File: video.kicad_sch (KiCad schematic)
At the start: 22 parts, among them J2 DIN-7 Video, J3 DIN-5 Audio, J4 DIN-5 Power, Q1 BC547B, Q3 BC547B, Q4 BC547B, Q5 BC547B, Q6 BC547B

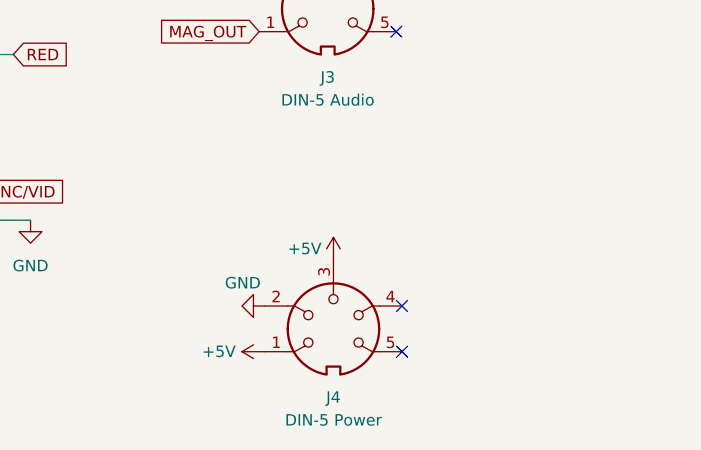
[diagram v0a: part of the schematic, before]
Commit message: Version 1.2 update
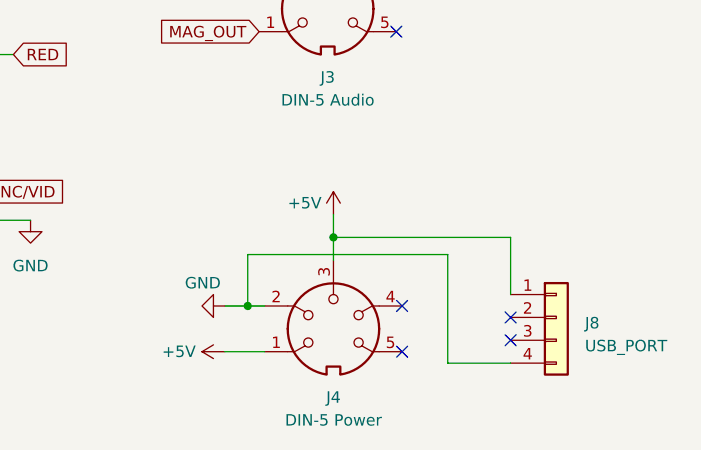
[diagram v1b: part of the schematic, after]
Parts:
- added J8: USB_PORT, Connector_PinHeader_2.54mm:PinHeader_1x04_P2.54mm_Vertical, symbol Connector_Generic:Conn_01x04
- J2: footprint w_conn_av:DIN-7-Variable -> Delta_sm_lib:DIN-7-Variable
- J3, J4: footprint w_conn_av:DIN-5-Variable -> Delta_sm_lib:DIN-5-Variable
- JP6: footprint Connector_PinHeader_2.54mm:PinHeader_2x03_P2.54mm_Vertical -> Delta_sm_lib:PinHeader_2x03_P2.54mm_Vertical
- LS1: footprint delta:ZM-Piezo Buzzer-2207T2 -> Delta_sm_lib:ZM-Piezo Buzzer-2207T2
- Q1, Q3, Q4, Q5, Q6: footprint Package_TO_SOT_THT:TO-92_Inline -> Delta_sm_lib:TO-92_Inline
- R24, R25, R26, R28, R30, R33, R37, R40, R7: footprint Resistor_THT:R_Axial_DIN0207_L6.3mm_D2.5mm_P10.16mm_Horizontal -> Delta_sm_lib:R_Axial_DIN0207_L6.3mm_D2.5mm_P10.16mm_Horizontal
- RV42, RV43, RV44: footprint Potentiometer_THT:Potentiometer_Bourns_3299X_Horizontal -> Delta_sm_lib:Potentiometer_Bourns_3299X_Horizontal
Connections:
- net +5V: now also J8.1 (Pin_1)
- net GND: now also J8.4 (Pin_4)
- no-connect marks 4 -> 6

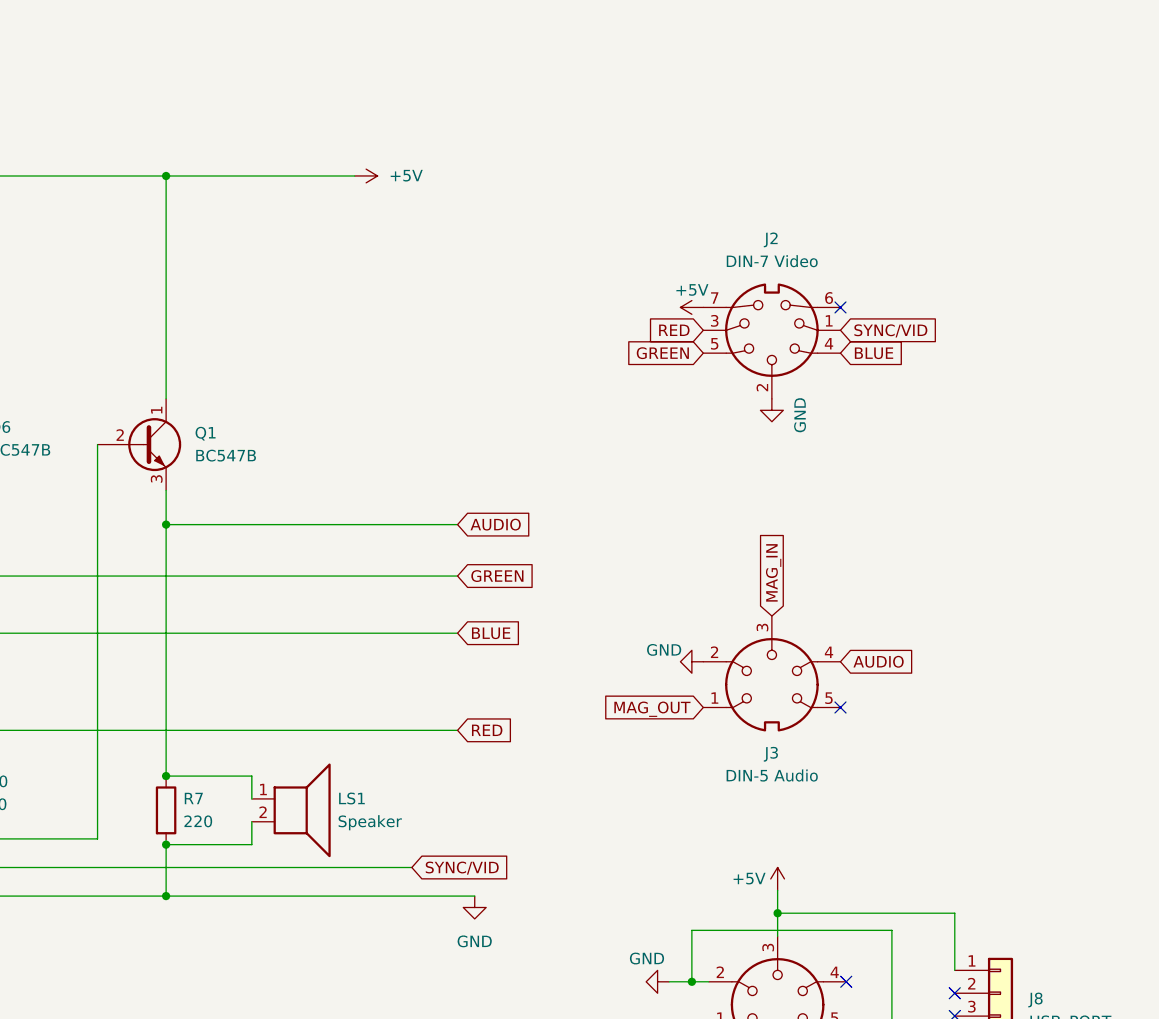
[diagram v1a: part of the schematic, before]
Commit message: Update 1.2, additional pins
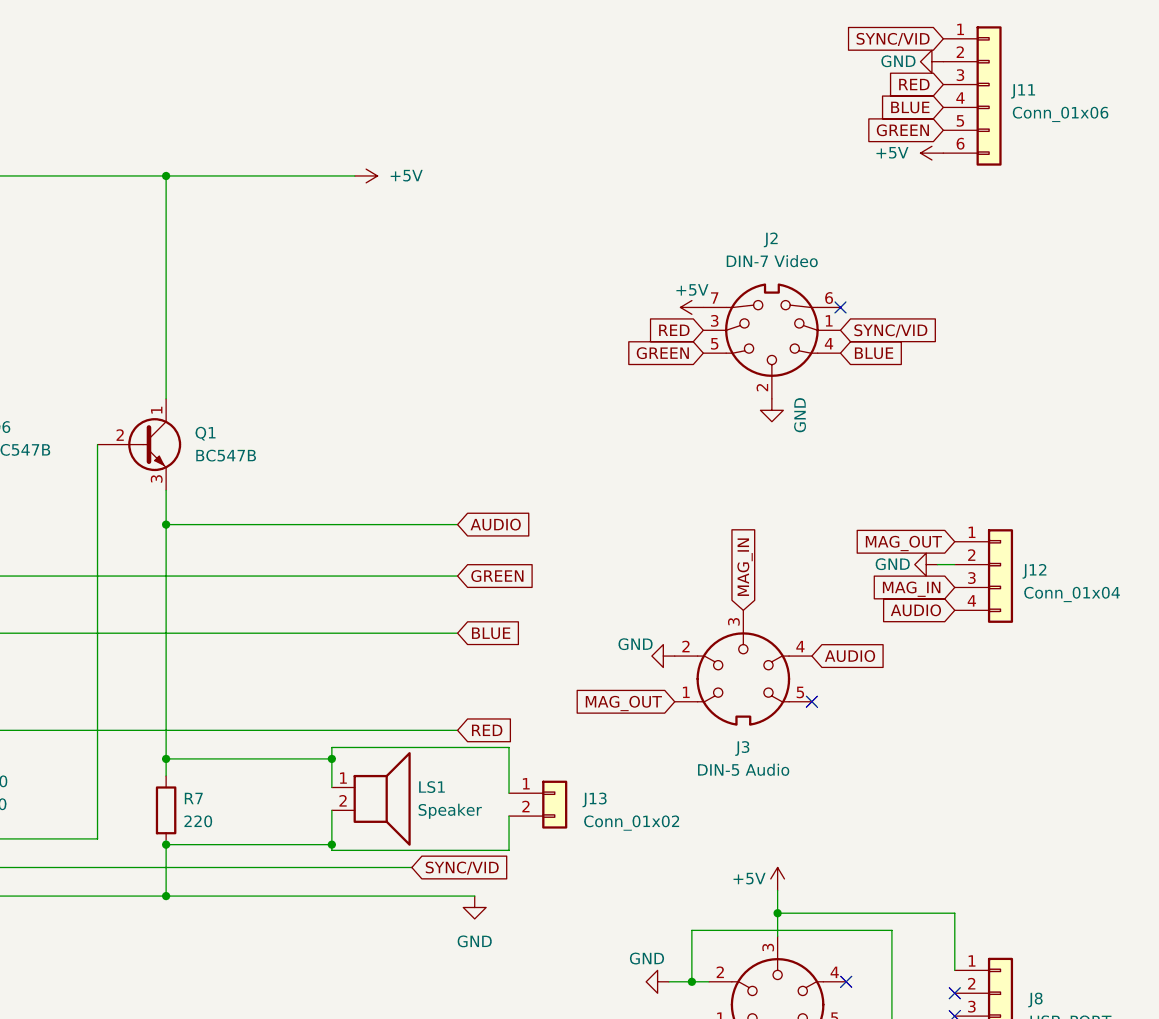
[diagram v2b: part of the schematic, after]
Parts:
- added J11: Conn_01x06, Connector_PinHeader_2.54mm:PinHeader_1x06_P2.54mm_Vertical, symbol Connector_Generic:Conn_01x06
- added J12: Conn_01x04, Connector_PinHeader_2.54mm:PinHeader_1x04_P2.54mm_Vertical, symbol Connector_Generic:Conn_01x04
- added J13: Conn_01x02, Connector_PinHeader_2.54mm:PinHeader_1x02_P2.54mm_Vertical, symbol Connector_Generic:Conn_01x02
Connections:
- net +5V: now also J11.6 (Pin_6)
- net AUDIO: now also J12.4 (Pin_4), J13.1 (Pin_1)
- net BLUE: now also J11.4 (Pin_4)
- net GND: now also J11.2 (Pin_2), J12.2 (Pin_2), J13.2 (Pin_2)
- net GREEN: now also J11.5 (Pin_5)
- net MAG_IN: now also J12.3 (Pin_3)
- net MAG_OUT: now also J12.1 (Pin_1)
- net RED: now also J11.3 (Pin_3)
- net SYNC/VID: now also J11.1 (Pin_1)
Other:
- moved on the sheet: J3, LS1

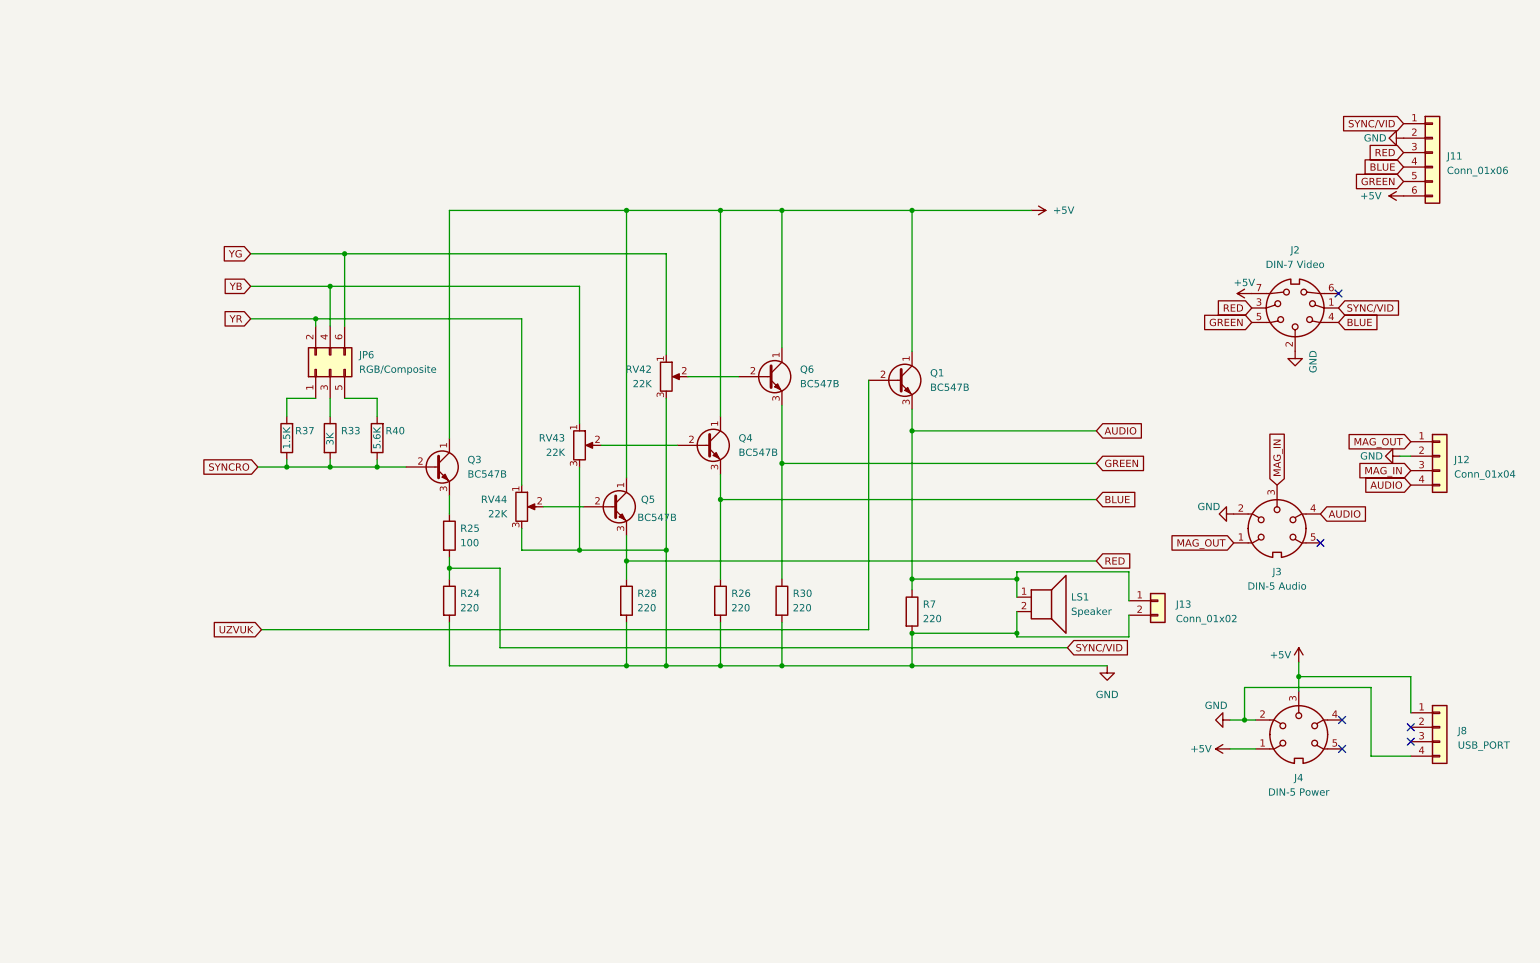
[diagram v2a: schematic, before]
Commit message: Topology for version 1.2
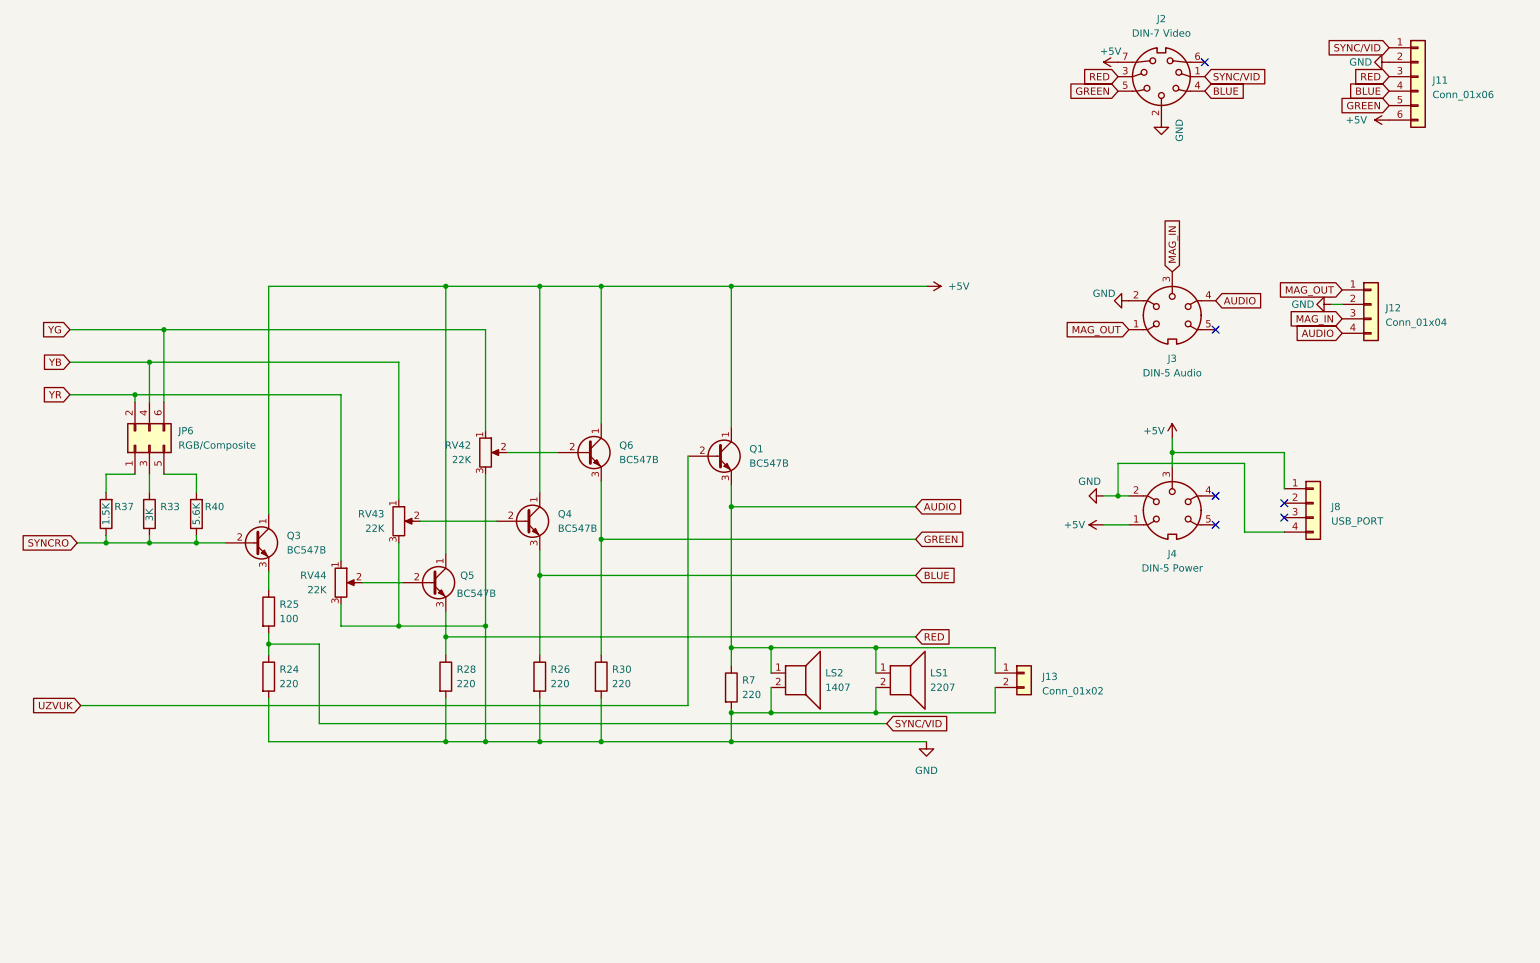
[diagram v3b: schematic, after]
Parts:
- added LS2: 1407, Delta_sm_lib:1407 Piezoelectric Passive Buzzer, symbol Delta_s_m_Lib:Speaker
- J8: footprint Connector_PinHeader_2.54mm:PinHeader_1x04_P2.54mm_Vertical -> Delta_sm_lib:USB-C Power board
- LS1: value Speaker -> 2207
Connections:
- net AUDIO: now also LS2.1
- net GND: now also LS2.2
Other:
- moved on the sheet: J11, J12, J13, J2, J3, J4, J8, JP6, LS1, Q1, Q3, Q4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

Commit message: Fixes
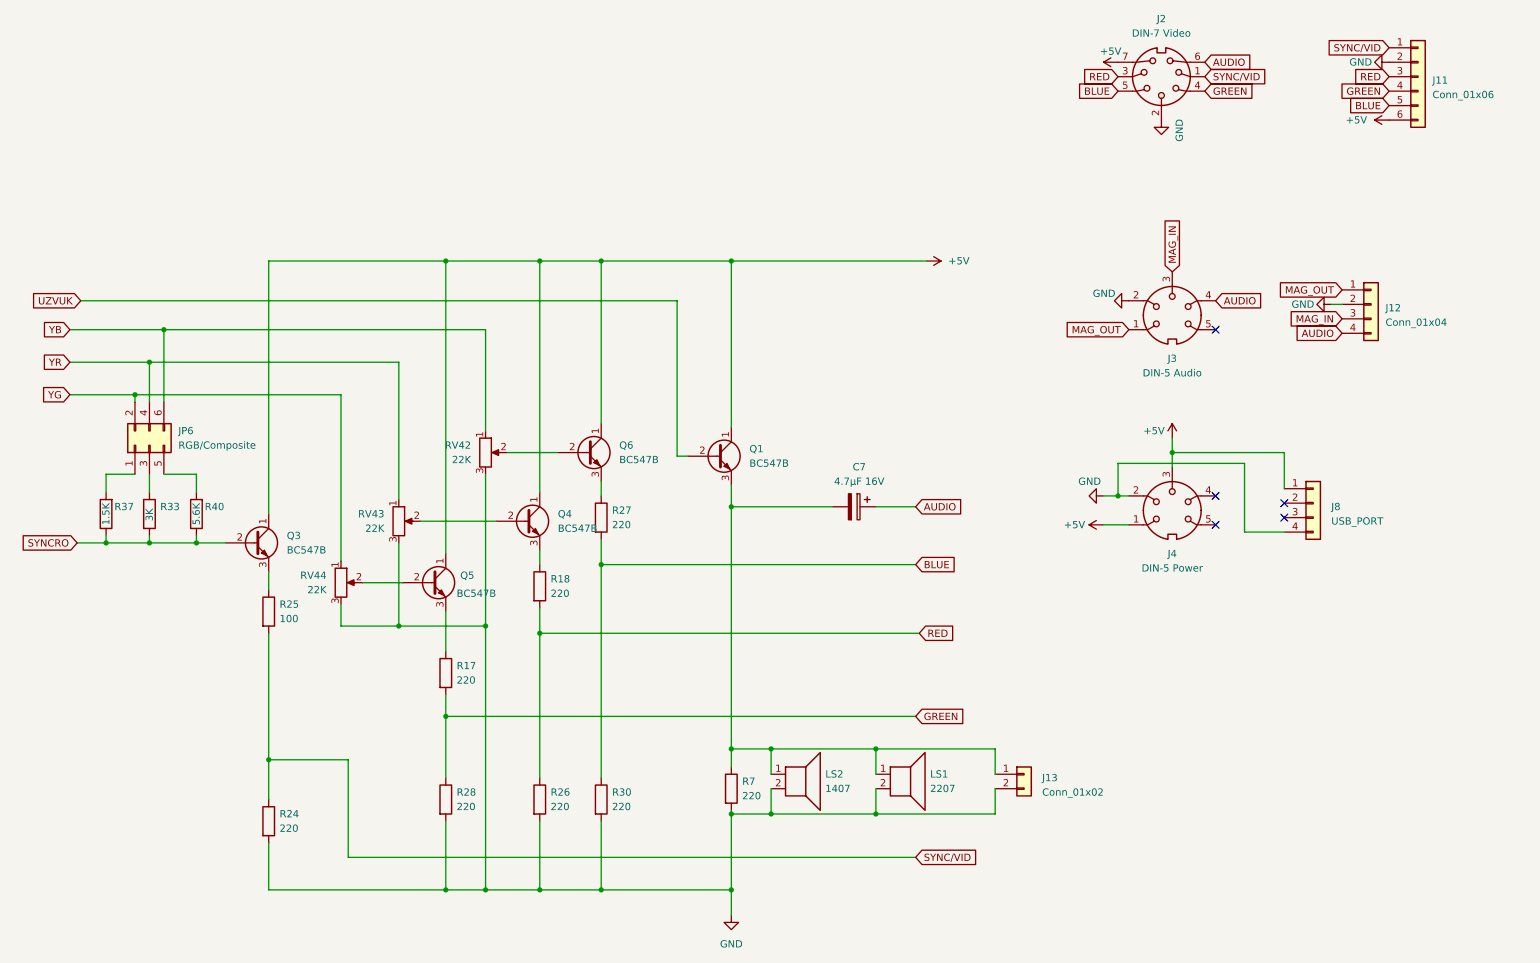
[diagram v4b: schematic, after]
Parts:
- added C7: 4.7µF 16V, Delta_sm_lib:CP_Radial_D4.0mm_P2.00mm, symbol Delta_s_m_Lib:C_Polarized
- added R17, R18, R27: 220, Delta_sm_lib:R_Axial_DIN0207_L6.3mm_D2.5mm_P10.16mm_Horizontal, symbol Delta_s_m_Lib:R
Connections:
- net AUDIO: now also J2.6, C7.1; no longer J13.1 (Pin_1), LS1.1, LS2.1, Q1.3 (E), R7.1
- net BLUE: now also J11.5 (Pin_5), J2.5, R30.1, R27.2; no longer J11.4 (Pin_4), J2.4, Q4.3 (E), R26.1
- net GREEN: now also J11.4 (Pin_4), J2.4, R28.1, R17.2; no longer J11.5 (Pin_5), J2.5, Q6.3 (E), R30.1
- net RED: now also R26.1, R18.2; no longer Q5.3 (E), R28.1
- net YB: now also JP6.6 (Pin_6), RV42.1; no longer JP6.4 (Pin_4), RV43.1
- net YG: now also JP6.2 (Pin_2), RV44.1; no longer JP6.6 (Pin_6), RV42.1
- net YR: now also JP6.4 (Pin_4), RV43.1; no longer JP6.2 (Pin_2), RV44.1
- new net: C7.2, J13.1 (Pin_1), LS1.1, LS2.1, Q1.3 (E), R7.1
- new net: Q4.3 (E), R18.1
- new net: Q6.3 (E), R27.1
- new net: Q5.3 (E), R17.1
- no-connect marks 6 -> 5
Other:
- moved on the sheet: J13, LS1, LS2, R24, R26, R28, R30, R7
